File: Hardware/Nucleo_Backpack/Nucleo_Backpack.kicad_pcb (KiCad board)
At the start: 2 copper layers, 70 x 57.5 mm, 48 parts, among them J1 CN7, J2 CN10, J4 Conn_01x04, J5 MEM2067-02-180-00-A_REVB, U3 ADXL375, U4 BMP390, U6 BMI323, U9 LR62E

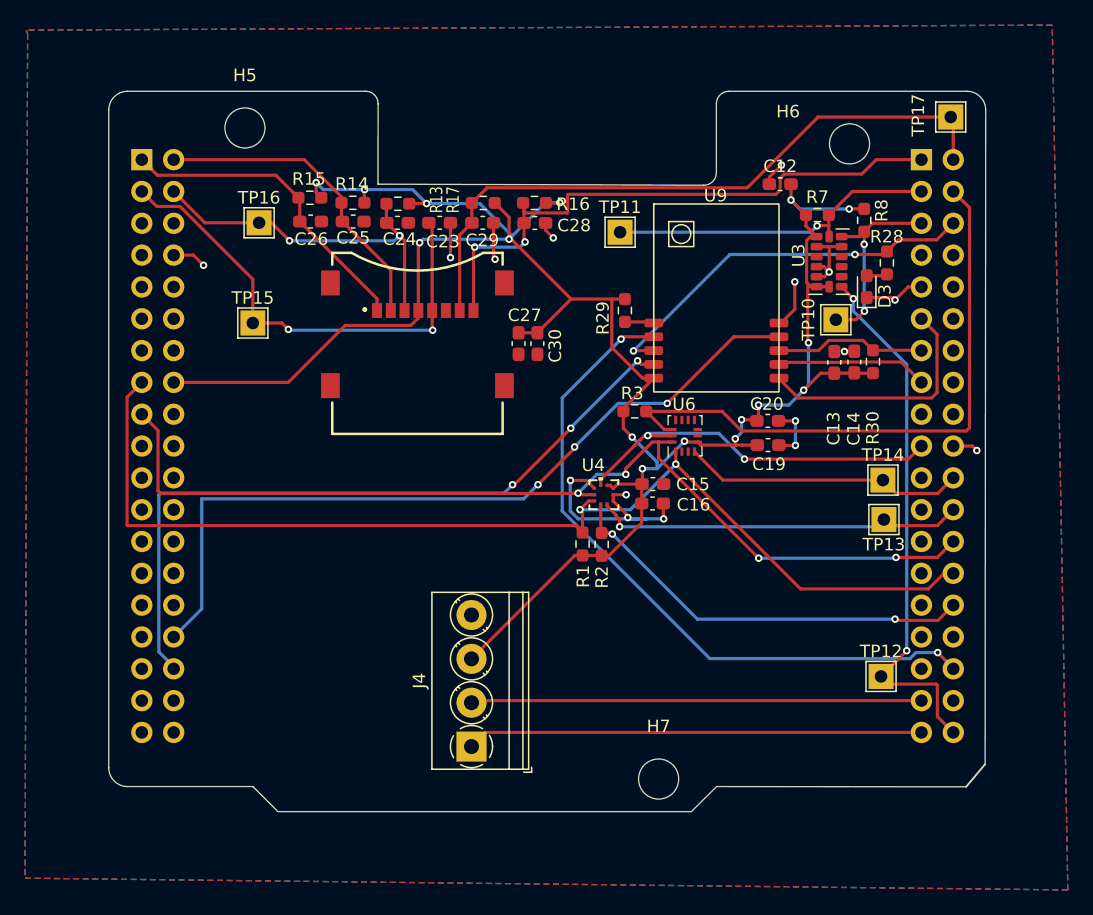
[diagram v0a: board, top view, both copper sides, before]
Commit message: cleaned up boards
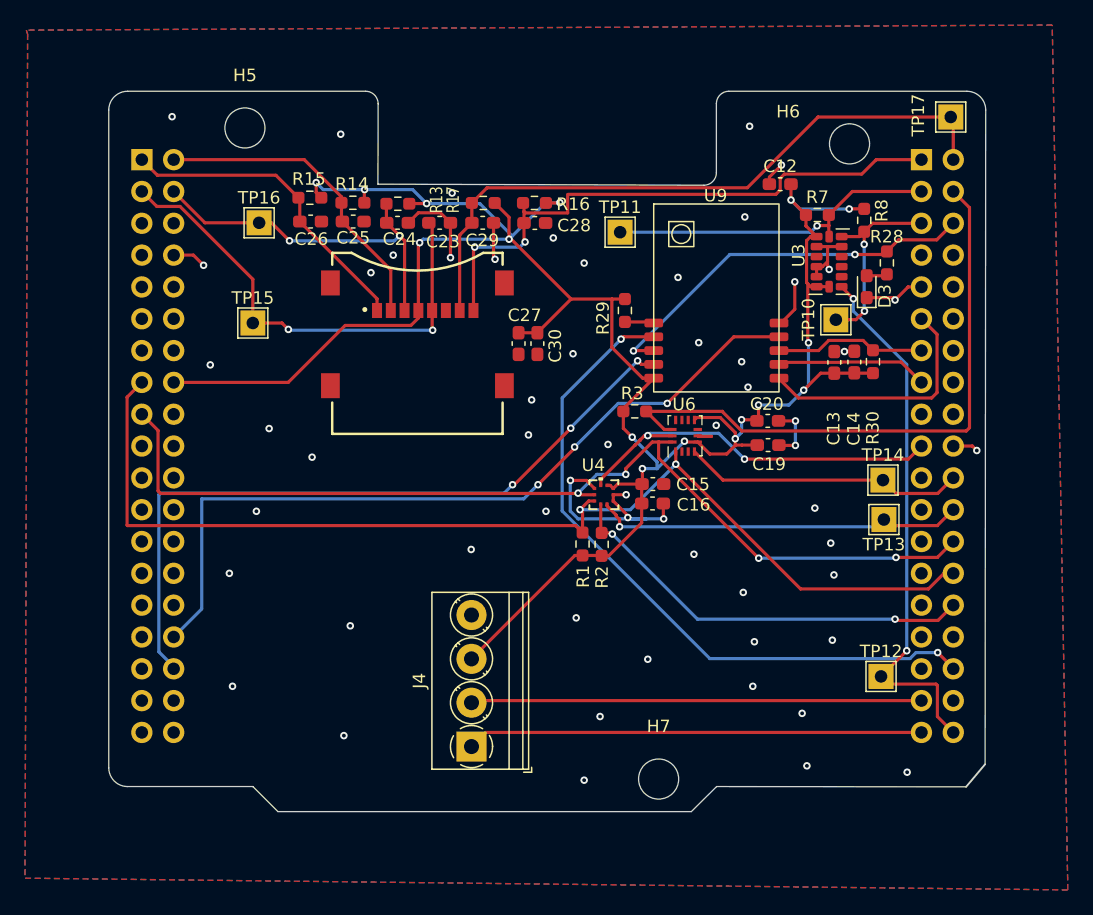
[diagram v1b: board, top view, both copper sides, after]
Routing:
- net +3.3V: track 177.3 -> 182.2 mm
- net GND: track 53.9 -> 56.0 mm, vias 16 -> 58

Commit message: regenerate gerbers
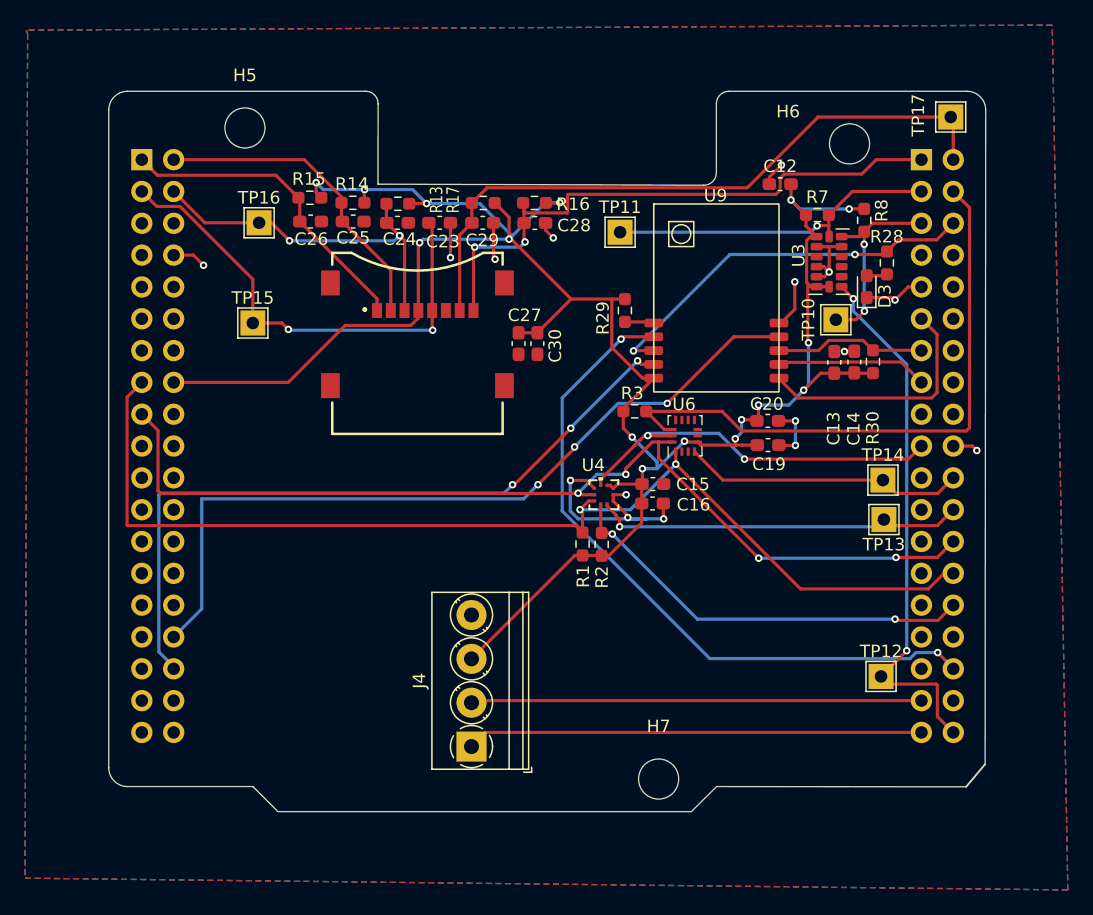
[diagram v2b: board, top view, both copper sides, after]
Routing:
- net +3.3V: track 182.2 -> 177.3 mm
- net GND: track 56.0 -> 53.9 mm, vias 58 -> 16
